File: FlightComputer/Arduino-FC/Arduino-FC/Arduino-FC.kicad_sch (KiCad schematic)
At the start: 30 parts, among them J1 Conn_01x04, J2 Conn_01x08, J3 Conn_01x06, J4 Conn_01x03, J5 Screw_Terminal_01x02, J6 Conn_01x02, J7 Conn_01x02, U1 NRF24L01_Breakout

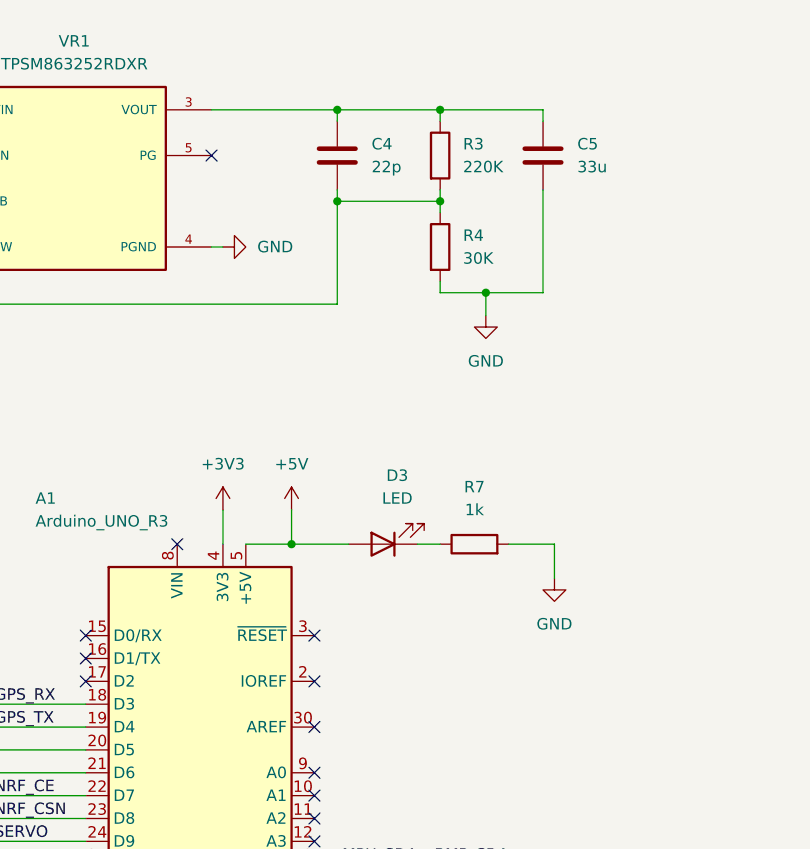
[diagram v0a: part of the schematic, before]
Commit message: Major Layout + Logo
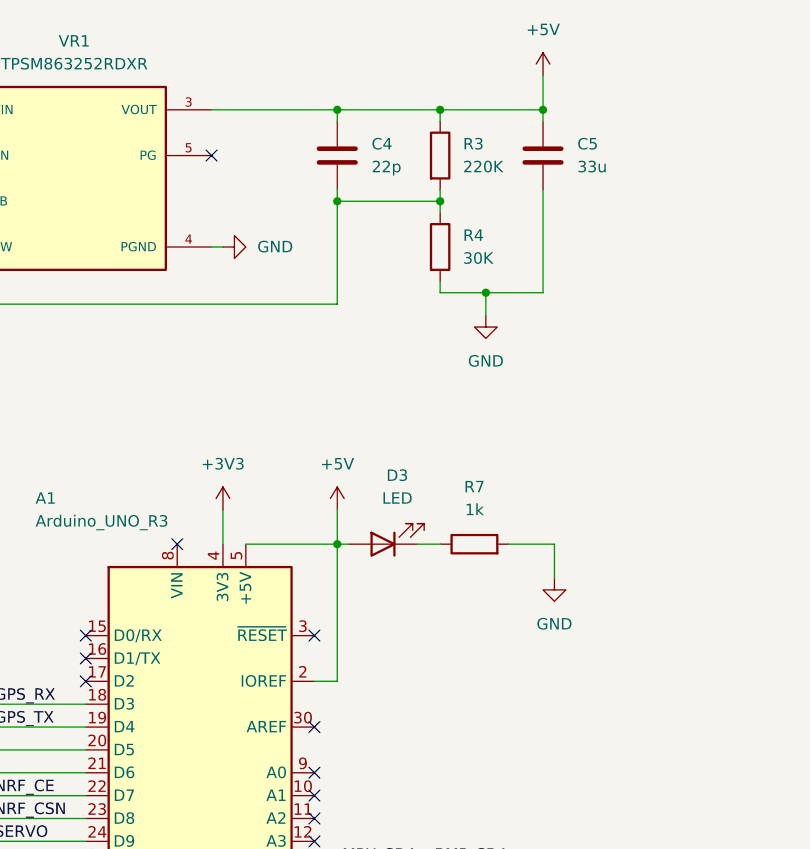
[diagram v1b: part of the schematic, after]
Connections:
- net +5V: now also A1.2 (IOREF), C4.1, C5.1, R3.1, VR1.3 (VOUT)
- no-connect marks 23 -> 22
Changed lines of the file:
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@@
 	(title_block
 		(title "Arduino Flight Computer")
-		(date "2026-04-30")
+		(date "2026-05-26")
 		(rev "v1.0")
 		(company "Team 'Lite Work: CANSAT STEC Initiative")
@@
 	)
 	(junction
+		(at 176.53 26.67)
+		(diameter 0)
+		(color 0 0 0 0)
+	)
+	(junction
 		(at 138.43 129.54)
 		(diameter 0)
@@
 	)
 	(junction
-		(at 148.59 74.93)
-		(diameter 0)
-		(color 0 0 0 0)
-	)
-	(junction
 		(at 82.55 50.8)
 		(diameter 0)
@@
 		(color 0 0 0 0)
 	)
+	(junction
+		(at 153.67 74.93)
+		(diameter 0)
+		(color 0 0 0 0)
+	)
 	(no_connect
 		(at 227.33 104.14)
@@
 	)
 	(no_connect
-		(at 151.13 90.17)
-	)
-	(no_connect
 		(at 125.73 110.49)
 	)
@@
 	(wire
 		(pts
+			(xy 153.67 74.93) (xy 154.94 74.93)
+		)
+		(stroke
+			(width 0)
+			(type default)
+		)
+	)
+	(wire
+		(pts
 			(xy 170.18 46.99) (xy 170.18 49.53)
 		)
@@
 	(wire
 		(pts
-			(xy 143.51 74.93) (xy 148.59 74.93)
+			(xy 143.51 74.93) (xy 153.67 74.93)
 		)
 		(stroke
@@
 	(wire
 		(pts
-			(xy 148.59 74.93) (xy 154.94 74.93)
-		)
-		(stroke
-			(width 0)
-			(type default)
-		)
-	)
-	(wire
-		(pts
 			(xy 66.04 38.1) (xy 71.12 38.1)
 		)
@@
 	(wire
 		(pts
+			(xy 176.53 22.86) (xy 176.53 26.67)
+		)
+		(stroke
+			(width 0)
+			(type default)
+		)
+	)
+	(wire
+		(pts
 			(xy 217.17 46.99) (xy 227.33 46.99)
 		)
@@
 	(wire
 		(pts
+			(xy 151.13 90.17) (xy 153.67 90.17)
+		)
+		(stroke
+			(width 0)
+			(type default)
+		)
+	)
+	(wire
+		(pts
 			(xy 71.12 26.67) (xy 71.12 29.21)
 		)
@@
 	(wire
 		(pts
+			(xy 153.67 90.17) (xy 153.67 74.93)
+		)
+		(stroke
+			(width 0)
+			(type default)
+		)
+	)
+	(wire
+		(pts
 			(xy 217.17 54.61) (xy 227.33 54.61)
 		)
@@
 	(wire
 		(pts
-			(xy 148.59 74.93) (xy 148.59 71.12)
+			(xy 153.67 74.93) (xy 153.67 71.12)
 		)
 		(stroke
@@
 	(symbol
 		(lib_id "power:+5V")
-		(at 148.59 71.12 0)
+		(at 153.67 71.12 0)
 		(unit 1)
 		(exclude_from_sim no)
@@
 		(fields_autoplaced yes)
 		(property "Reference" "#PWR011"
-			(at 148.59 74.93 0)
+			(at 153.67 74.93 0)
 			(effects
 				(font
@@
 		)
 		(property "Value" "+5V"
-			(at 148.59 66.04 0)
+			(at 153.67 66.04 0)
 			(effects
 				(font
@@
 		)
 		(property "Footprint" ""
-			(at 148.59 71.12 0)
+			(at 153.67 71.12 0)
 			(effects
 				(font
@@
 		)
 		(property "Datasheet" ""
-			(at 148.59 71.12 0)
+			(at 153.67 71.12 0)
 			(effects
 				(font
@@
 		)
 		(property "Description" "Power symbol creates a global label with name \"+5V\""
-			(at 148.59 71.12 0)
+			(at 153.67 71.12 0)
 			(effects
 				(font
@@
 					(unit 1)
 				)
+			)
+		)
+	)
+	(symbol
+		(lib_id "power:+5V")
+		(at 176.53 22.86 0)
+		(unit 1)
+		(exclude_from_sim no)
+		(in_bom yes)
+		(on_board yes)
+		(dnp no)
+		(fields_autoplaced yes)
+		(property "Reference" "#PWR022"
+			(at 176.53 26.67 0)
+			(effects
+				(font
+					(size 1.27 1.27)
+				)
+				(hide yes)
+			)
+		)
+		(property "Value" "+5V"
+			(at 176.53 17.78 0)
+			(effects
+				(font
+					(size 1.27 1.27)
+				)
+			)
+		)
+		(property "Footprint" ""
+			(at 176.53 22.86 0)
+			(effects
+				(font
+					(size 1.27 1.27)
+				)
+				(hide yes)
+			)
+		)
+		(property "Datasheet" ""
+			(at 176.53 22.86 0)
+			(effects
+				(font
+					(size 1.27 1.27)
+				)
+				(hide yes)
+			)
+		)
+		(property "Description" "Power symbol creates a global label with name \"+5V\""
+			(at 176.53 22.86 0)
+			(effects
+				(font
+					(size 1.27 1.27)
+				)
+				(hide yes)
+			)
+		)
+		(pin "1"
+		)
+		(instances
+			(project "Arduino-FC"
+				(path "/979d3eec-a24a-4073-bdb5-1e3cad04034a"
+					(reference "#PWR022")
+					(unit 1)
+				)
